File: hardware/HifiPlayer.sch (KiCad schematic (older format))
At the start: 9 parts, among them J1 Conn_01x04_Male, J2 Conn_01x03_Male, J3 Conn_01x06_Male, J4 Screw_Terminal_01x03, J5 Conn_01x02_Male, U1 STM32G071KBTx

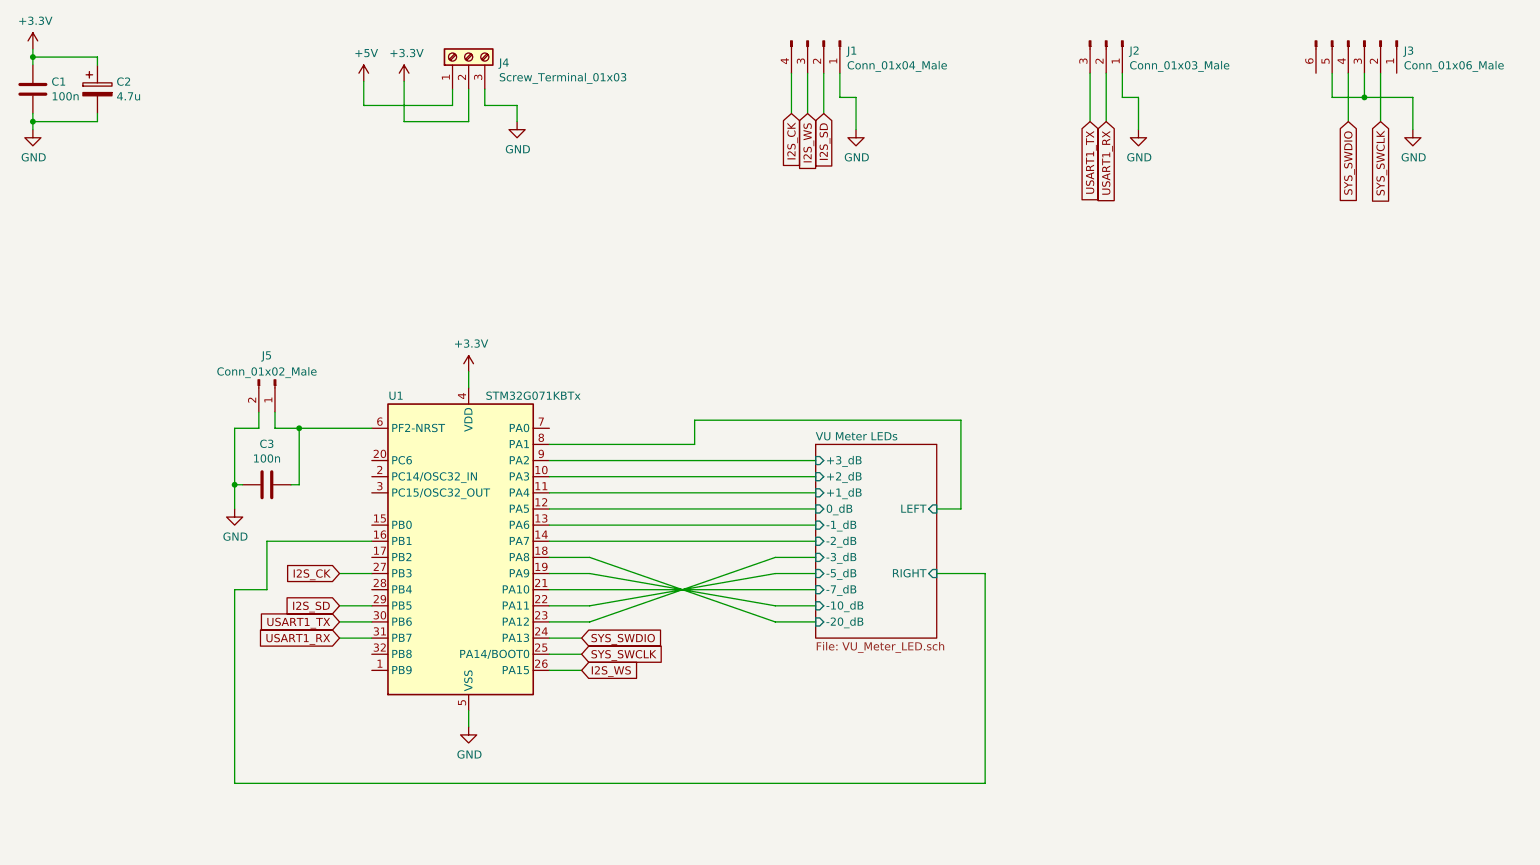
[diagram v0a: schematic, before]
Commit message: Finished PCD Mk.1
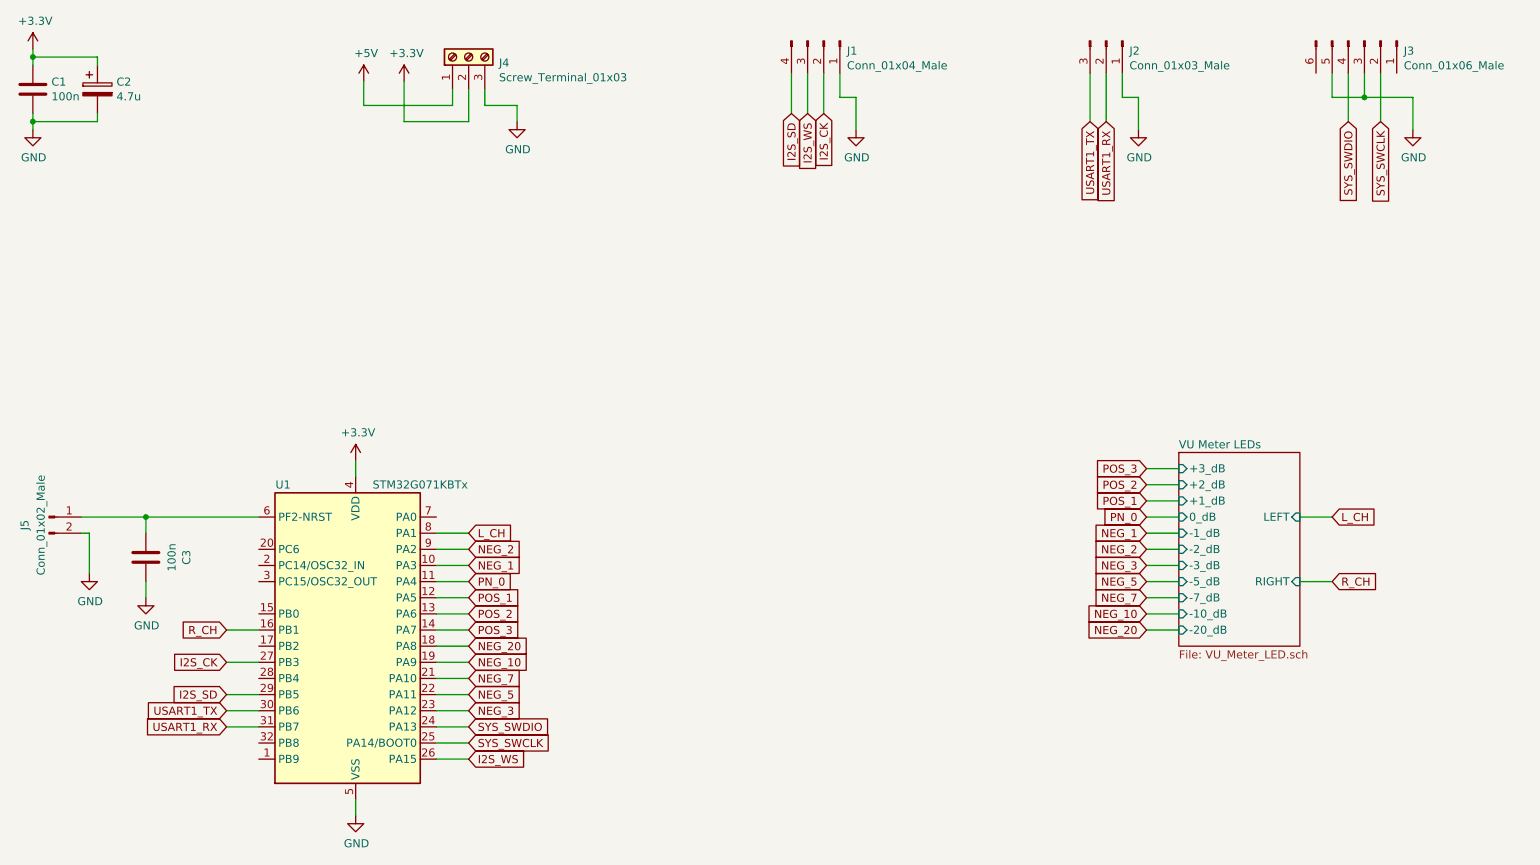
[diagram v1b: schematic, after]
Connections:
- net GND: now also C3.1; no longer C3.2
- net I2S_CK: now also J1.2 (Pin_2); no longer J1.4 (Pin_4)
- net I2S_SD: now also J1.4 (Pin_4); no longer J1.2 (Pin_2)
- net at J5.1 (Pin_1), U1.6 (PF2-NRST): now also C3.2; no longer C3.1
- net VU Meter LEDs/+1_dB renamed PN_0
- net VU Meter LEDs/+2_dB renamed NEG_1
- net VU Meter LEDs/+3_dB renamed NEG_2
- net VU Meter LEDs/-10_dB renamed NEG_10
- net VU Meter LEDs/-1_dB renamed POS_2
- net VU Meter LEDs/-20_dB renamed NEG_20
- net VU Meter LEDs/-2_dB renamed POS_3
- net VU Meter LEDs/-3_dB renamed NEG_3
- net VU Meter LEDs/-5_dB renamed NEG_5
- net VU Meter LEDs/-7_dB renamed NEG_7
- net VU Meter LEDs/0_dB renamed POS_1
- net VU Meter LEDs/LEFT renamed L_CH
- net VU Meter LEDs/RIGHT renamed R_CH
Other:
- moved on the sheet: C3, J5, U1
